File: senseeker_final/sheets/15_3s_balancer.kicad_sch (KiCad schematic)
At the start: 32 parts, among them J1 Conn_01x02, J4 Conn_01x04, Q1 AO4892, Q2 BSS84, SW1 TS-1088R-02026, U1 NTC10K/0805/F, U4 BQ76920PW

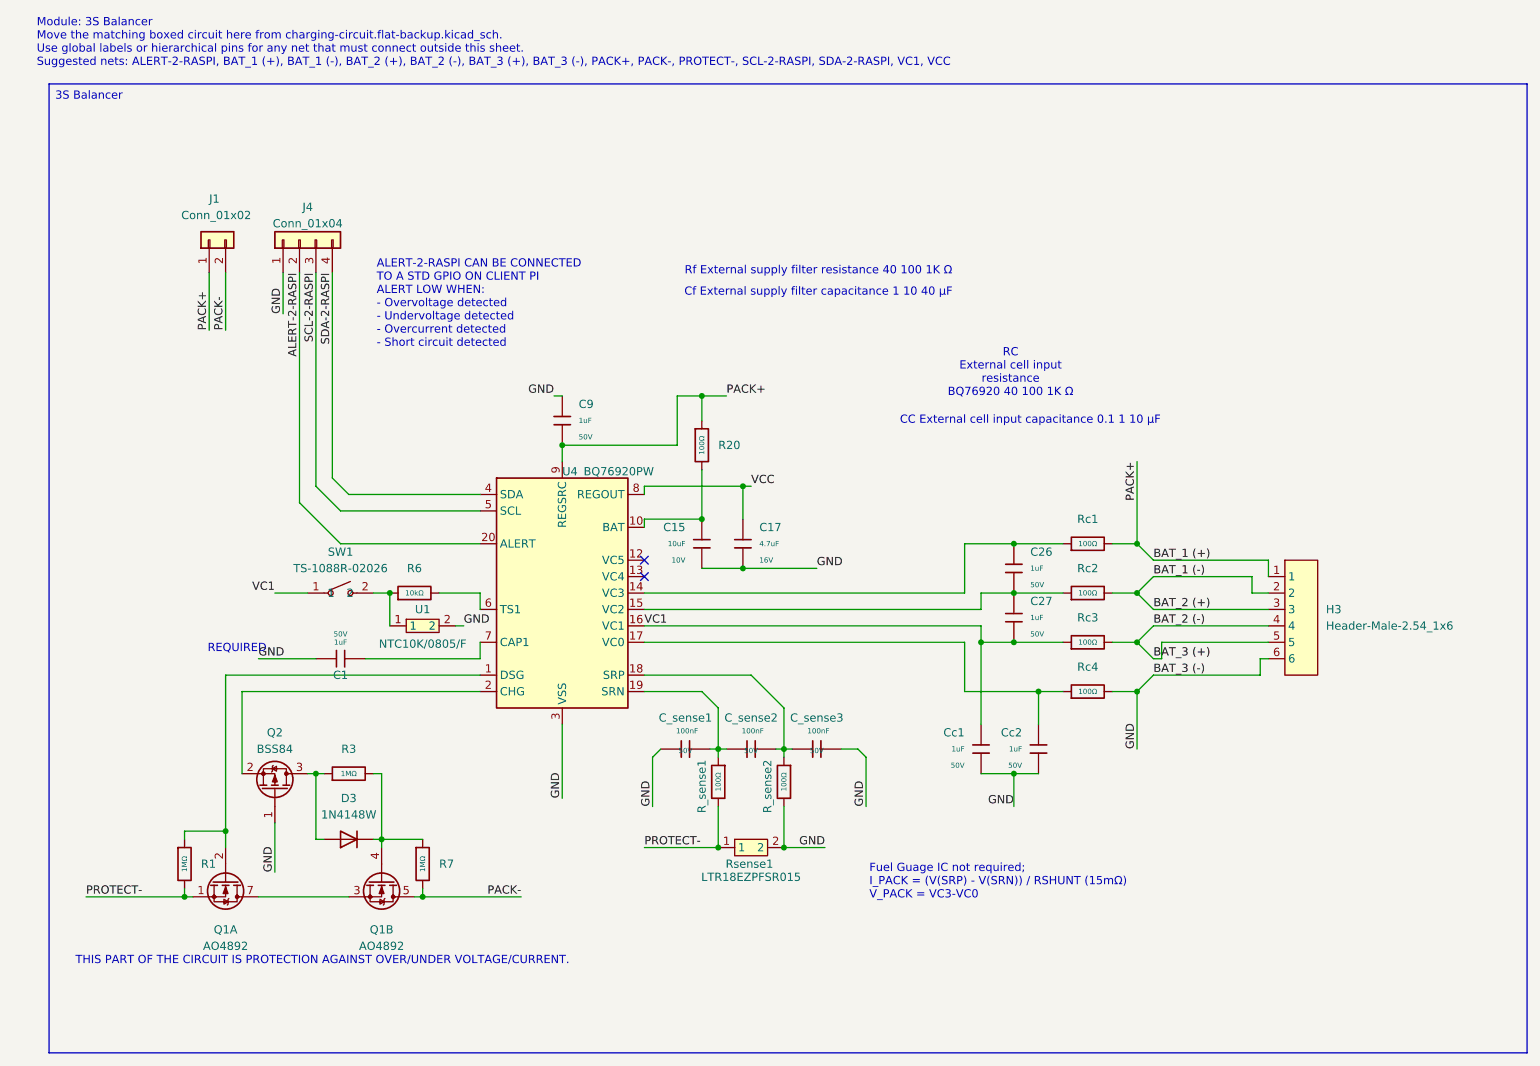
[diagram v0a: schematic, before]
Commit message: finished for tn
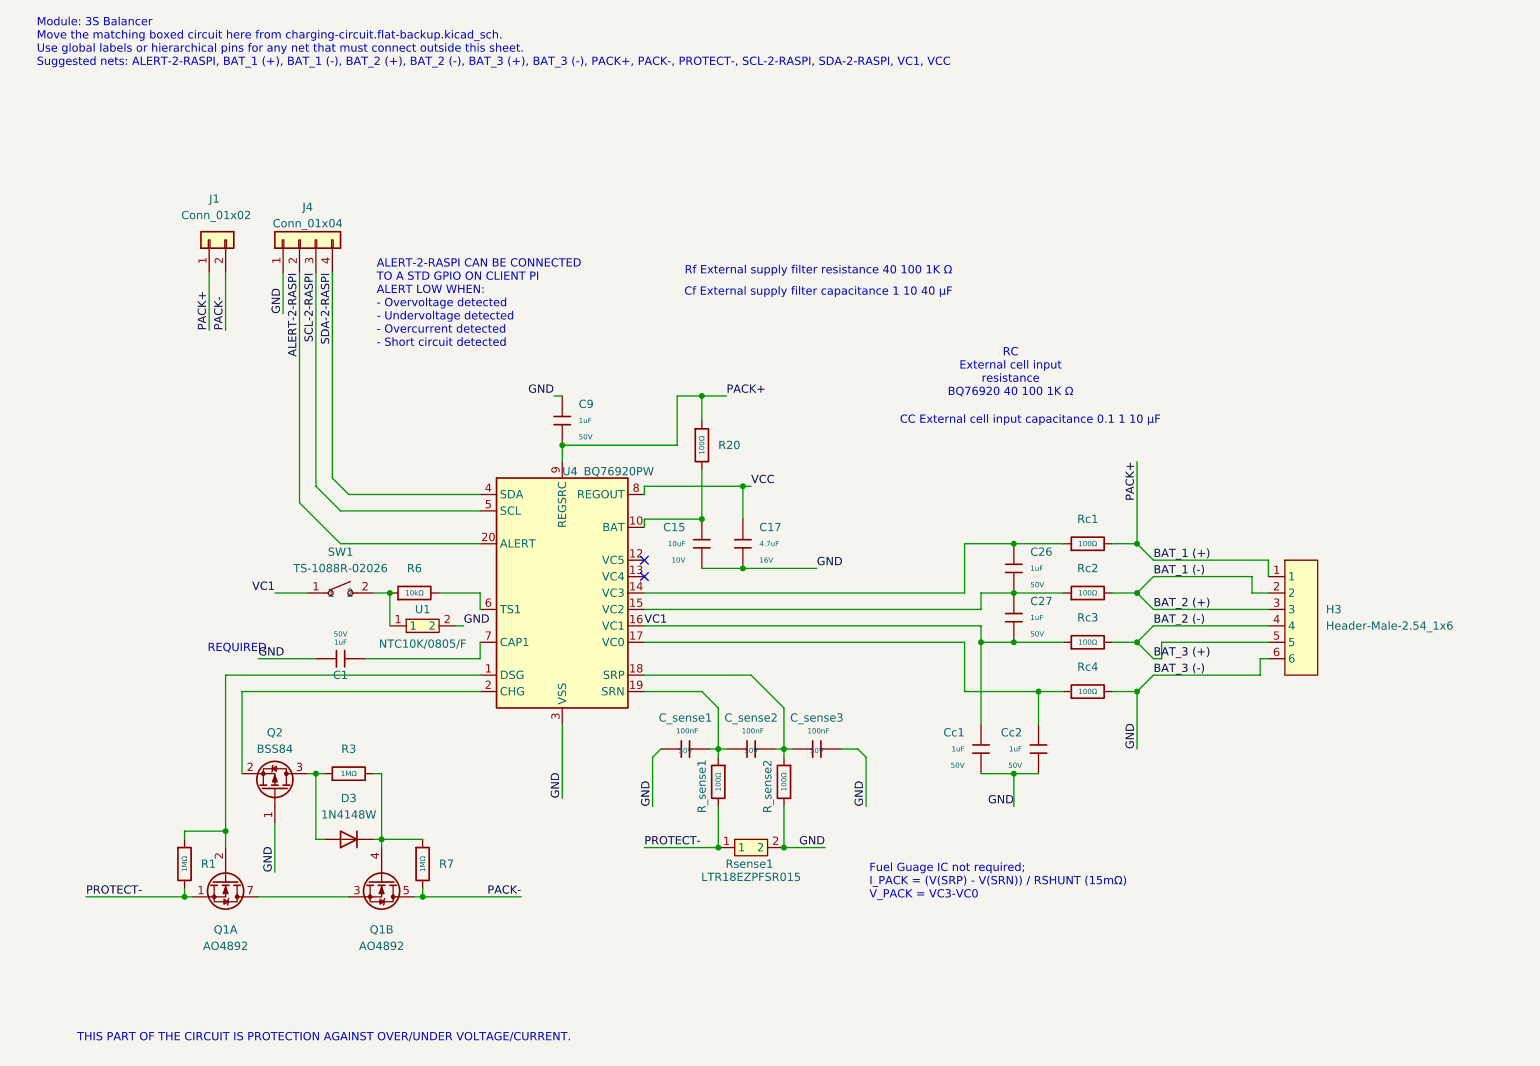
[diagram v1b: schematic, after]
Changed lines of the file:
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@@
 	(text "THIS PART OF THE CIRCUIT IS PROTECTION AGAINST OVER/UNDER VOLTAGE/CURRENT."
 		(exclude_from_sim no)
-		(at 69.596 167.386 0)
+		(at 69.85 179.324 0)
 		(effects
 			(font
@@
 		)
 	)
-	(text_box "3S Balancer\n"
-		(exclude_from_sim no)
-		(at 27.305 31.75 0)
-		(size 228.6 149.86)
-		(margins 0.9525 0.9525 0.9525 0.9525)
-		(stroke
-			(width 0)
-			(type solid)
-		)
-		(fill
-			(type none)
-		)
-		(effects
-			(font
-				(size 1.27 1.27)
-			)
-			(justify left top)
-		)
-	)
